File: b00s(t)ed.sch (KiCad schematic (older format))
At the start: 1 part, among them Q1 IRL7472L1

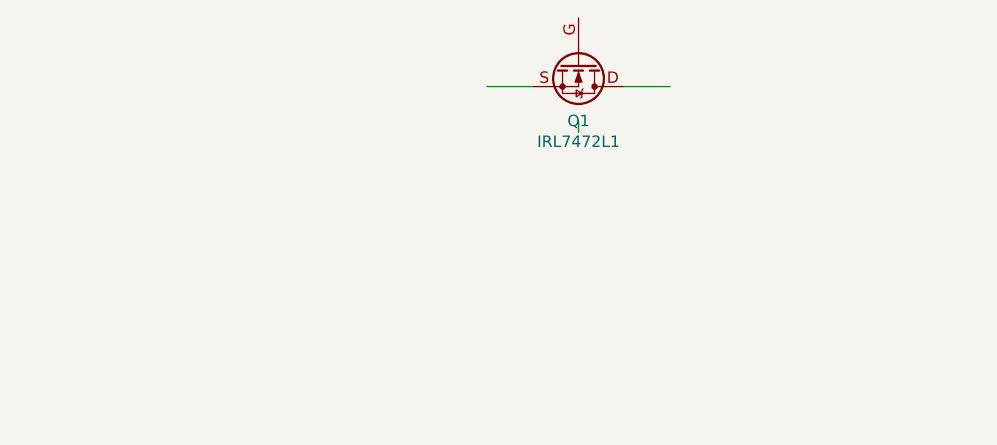
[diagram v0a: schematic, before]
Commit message: backup
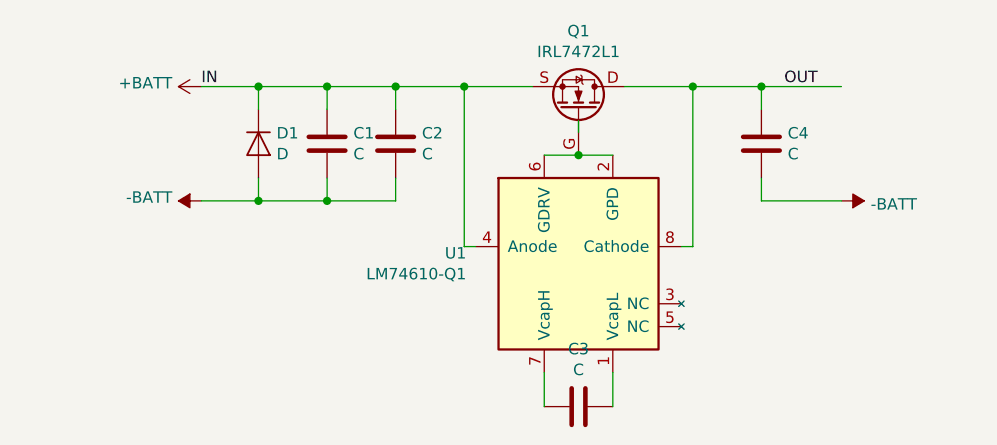
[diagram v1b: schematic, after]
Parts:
- added C1, C2, C3, C4: C, Capacitor_SMD:C_1206_3216Metric, symbol Device:C
- added D1: D, Diode_SMD:D_SMB, symbol Device:D
- added U1: LM74610-Q1, Package_SO:S-PDSO-G8, symbol Power_Management:LM74610-Q1
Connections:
- net labels added: +BATT, -BATT, IN, OUT
- wire segments 3 -> 29
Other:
- moved on the sheet: Q1
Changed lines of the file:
@@
 $EndDescr
 Wire Wire Line
-	5700 2400 5500 2400
+	5700 2400 5400 2400
 Wire Wire Line
 	5900 2600 5900 2550
@@
 L Transistor_FET:IRL7472L1 Q1
 U 1 1 5C52EA7D
-P 5900 2300
-F 0 "Q1" V 6150 2300 50  0000 C CNN
-F 1 "IRL7472L1" V 6241 2300 50  0000 C CNN
-F 2 "Package_DirectFET:DirectFET_L8" H 5900 2300 50  0001 C CIN
-F 3 "https://www.infineon.com/dgdl/Infineon-IRL7472L1-DS-v02_00-EN.pdf?fileId=5546d46254e133b401555d17178250d8" H 5900 2300 50  0001 L CNN
-	1    5900 2300
+P 5900 2500
+F 0 "Q1" V 6243 2500 50  0000 C CNN
+F 1 "IRL7472L1" V 6152 2500 50  0000 C CNN
+F 2 "Package_DirectFET:DirectFET_L8" H 5900 2500 50  0001 C CIN
+F 3 "https://www.infineon.com/dgdl/Infineon-IRL7472L1-DS-v02_00-EN.pdf?fileId=5546d46254e133b401555d17178250d8" H 5900 2500 50  0001 L CNN
+	1    5900 2500
+	0    1    -1   0
+$EndComp
+Wire Wire Line
+	6100 2400 6400 2400
+Text Label 4250 2400 0    50   ~ 0
+IN
+Text Label 6800 2400 0    50   ~ 0
+OUT
+$Comp
+L Power_Management:LM74610-Q1 U1
+U 1 1 5C5374D8
+P 5900 2950
+F 0 "U1" H 5409 2771 50  0000 R CNN
+F 1 "LM74610-Q1" H 5409 2680 50  0000 R CNN
+F 2 "Package_SO:S-PDSO-G8" H 5900 2250 50  0001 C CIN
+F 3 "http://www.irf.com/product-info/datasheets/data/auips7111s.pdf" H 5900 3150 50  0001 C CNN
+	1    5900 2950
+	1    0    0    -1
+$EndComp
+Wire Wire Line
+	5450 3100 5400 3100
+Wire Wire Line
+	5400 3100 5400 2400
+Connection ~ 5400 2400
+Wire Wire Line
+	5400 2400 5100 2400
+Wire Wire Line
+	6350 3100 6400 3100
+Wire Wire Line
+	6400 3100 6400 2400
+Connection ~ 6400 2400
+Wire Wire Line
+	6400 2400 6700 2400
+Wire Wire Line
+	5750 2700 5900 2700
+Wire Wire Line
+	6050 2700 5900 2700
+Connection ~ 5900 2700
+$Comp
+L Device:C C3
+U 1 1 5C53C78F
+P 5900 3800
+F 0 "C3" V 5648 3800 50  0000 C CNN
+F 1 "C" V 5739 3800 50  0000 C CNN
+F 2 "Capacitor_SMD:C_1206_3216Metric" H 5938 3650 50  0001 C CNN
+F 3 "~" H 5900 3800 50  0001 C CNN
+	1    5900 3800
 	0    1    1    0
 $EndComp
 Wire Wire Line
-	6100 2400 6300 2400
+	6050 3650 6050 3800
+Wire Wire Line
+	5750 3650 5750 3800
+$Comp
+L Device:D D1
+U 1 1 5C53D25D
+P 4500 2650
+F 0 "D1" V 4454 2729 50  0000 L CNN
+F 1 "D" V 4545 2729 50  0000 L CNN
+F 2 "Diode_SMD:D_SMB" H 4500 2650 50  0001 C CNN
+F 3 "~" H 4500 2650 50  0001 C CNN
+	1    4500 2650
+	0    1    1    0
+$EndComp
+$Comp
+L Device:C C2
+U 1 1 5C53D3D8
+P 5100 2650
+F 0 "C2" H 5215 2696 50  0000 L CNN
+F 1 "C" H 5215 2605 50  0000 L CNN
+F 2 "Capacitor_SMD:C_1206_3216Metric" H 5138 2500 50  0001 C CNN
+F 3 "~" H 5100 2650 50  0001 C CNN
+	1    5100 2650
+	1    0    0    -1
+$EndComp
+Wire Wire Line
+	5100 2500 5100 2400
+Connection ~ 5100 2400
+Wire Wire Line
+	5100 2400 4800 2400
+Wire Wire Line
+	4800 2500 4800 2400
+Connection ~ 4800 2400
+Wire Wire Line
+	4800 2400 4500 2400
+$Comp
+L Device:C C4
+U 1 1 5C53E8AA
+P 6700 2650
+F 0 "C4" H 6815 2696 50  0000 L CNN
+F 1 "C" H 6815 2605 50  0000 L CNN
+F 2 "Capacitor_SMD:C_1206_3216Metric" H 6738 2500 50  0001 C CNN
+F 3 "~" H 6700 2650 50  0001 C CNN
+	1    6700 2650
+	1    0    0    -1
+$EndComp
+Wire Wire Line
+	6700 2900 6700 2800
+Wire Wire Line
+	6700 2500 6700 2400
+Connection ~ 6700 2400
+Wire Wire Line
+	6700 2400 7050 2400
+$Comp
+L Device:C C1
+U 1 1 5C54035D
+P 4800 2650
+F 0 "C1" H 4915 2696 50  0000 L CNN
+F 1 "C" H 4915 2605 50  0000 L CNN
+F 2 "Capacitor_SMD:C_1206_3216Metric" H 4838 2500 50  0001 C CNN
+F 3 "~" H 4800 2650 50  0001 C CNN
+	1    4800 2650
+	1    0    0    -1
+$EndComp
+Wire Wire Line
+	4500 2500 4500 2400
+Connection ~ 4500 2400
+Wire Wire Line
+	4500 2400 4250 2400
+$Comp
+L power:+BATT #PWR0101
+U 1 1 5C5419B9
+P 4250 2400
+F 0 "#PWR0101" H 4250 2250 50  0001 C CNN
+F 1 "+BATT" V 4265 2527 50  0000 L CNN
+F 2 "" H 4250 2400 50  0001 C CNN
+F 3 "" H 4250 2400 50  0001 C CNN
+	1    4250 2400
+	0    -1   -1   0
+$EndComp
+$Comp
+L power:-BATT #PWR0103
+U 1 1 5C54344F
+P 4250 2900
+F 0 "#PWR0103" H 4250 2750 50  0001 C CNN
+F 1 "-BATT" V 4265 3027 50  0000 L CNN
+F 2 "" H 4250 2900 50  0001 C CNN
+F 3 "" H 4250 2900 50  0001 C CNN
+	1    4250 2900
+	0    -1   -1   0
+$EndComp
+$Comp
+L power:-BATT #PWR0104
+U 1 1 5C544FA1
+P 7050 2900
+F 0 "#PWR0104" H 7050 2750 50  0001 C CNN
+F 1 "-BATT" V 7065 3028 50  0000 L CNN
+F 2 "" H 7050 2900 50  0001 C CNN
+F 3 "" H 7050 2900 50  0001 C CNN
+	1    7050 2900
+	0    1    1    0
+$EndComp
+Wire Wire Line
+	6700 2900 7050 2900
+Wire Wire Line
+	4250 2900 4500 2900
+Wire Wire Line
+	5100 2900 5100 2800
+Wire Wire Line
+	4800 2800 4800 2900
+Connection ~ 4800 2900
+Wire Wire Line
+	4800 2900 5100 2900
+Wire Wire Line
+	4500 2800 4500 2900
+Connection ~ 4500 2900
+Wire Wire Line
+	4500 2900 4800 2900
 $EndSCHEMATC

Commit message: First version ready for order
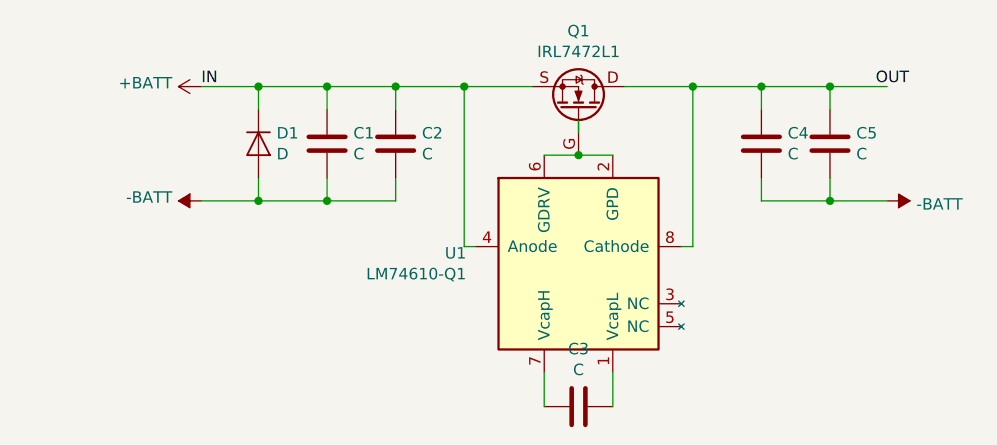
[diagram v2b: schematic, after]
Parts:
- added C5: C, Capacitor_SMD:C_1206_3216Metric, symbol Device:C
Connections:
- wire segments 29 -> 33
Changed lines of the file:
@@
 Text Label 4250 2400 0    50   ~ 0
 IN
-Text Label 6800 2400 0    50   ~ 0
+Text Label 7200 2400 0    50   ~ 0
 OUT
 $Comp
@@
 Connection ~ 6700 2400
 Wire Wire Line
-	6700 2400 7050 2400
+	6700 2400 7000 2400
 $Comp
 L Device:C C1
@@
 L power:-BATT #PWR0104
 U 1 1 5C544FA1
-P 7050 2900
-F 0 "#PWR0104" H 7050 2750 50  0001 C CNN
-F 1 "-BATT" V 7065 3028 50  0000 L CNN
-F 2 "" H 7050 2900 50  0001 C CNN
-F 3 "" H 7050 2900 50  0001 C CNN
-	1    7050 2900
+P 7250 2900
+F 0 "#PWR0104" H 7250 2750 50  0001 C CNN
+F 1 "-BATT" V 7265 3028 50  0000 L CNN
+F 2 "" H 7250 2900 50  0001 C CNN
+F 3 "" H 7250 2900 50  0001 C CNN
+	1    7250 2900
 	0    1    1    0
 $EndComp
 Wire Wire Line
-	6700 2900 7050 2900
+	6700 2900 7000 2900
 Wire Wire Line
 	4250 2900 4500 2900
@@
 Wire Wire Line
 	4500 2900 4800 2900
+$Comp
+L Device:C C5
+U 1 1 5C555923
+P 7000 2650
+F 0 "C5" H 7115 2696 50  0000 L CNN
+F 1 "C" H 7115 2605 50  0000 L CNN
+F 2 "Capacitor_SMD:C_1206_3216Metric" H 7038 2500 50  0001 C CNN
+F 3 "~" H 7000 2650 50  0001 C CNN
+	1    7000 2650
+	1    0    0    -1
+$EndComp
+Wire Wire Line
+	7000 2500 7000 2400
+Connection ~ 7000 2400
+Wire Wire Line
+	7000 2400 7250 2400
+Wire Wire Line
+	7000 2800 7000 2900
+Connection ~ 7000 2900
+Wire Wire Line
+	7000 2900 7250 2900
 $EndSCHEMATC

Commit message: ordered
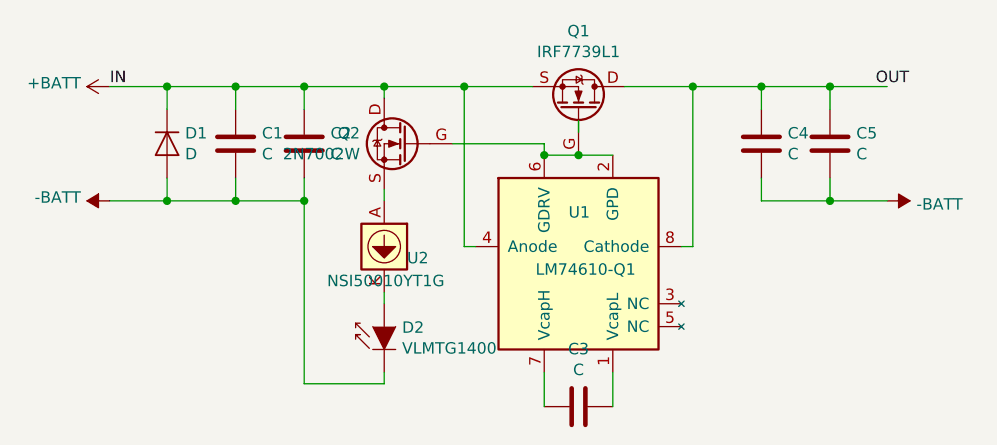
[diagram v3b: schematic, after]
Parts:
- added D2: VLMTG1400, Diode_SMD:D_0603_1608Metric, symbol LED:VLMTG1400
- added Q2: 2N7002W, Package_TO_SOT_SMD:SOT-323_SC-70, symbol Transistor_FET:2N7002W
- added U2: NSI50010YT1G, Digikey:SOD-123, symbol Regulator_Current:NSI50010YT1G
- Q1: value IRL7472L1 -> IRF7739L1
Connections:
- wire segments 33 -> 42
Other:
- moved on the sheet: C1, C2, D1
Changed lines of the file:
@@
 P 5900 2500
 F 0 "Q1" V 6243 2500 50  0000 C CNN
-F 1 "IRL7472L1" V 6152 2500 50  0000 C CNN
+F 1 "IRF7739L1" V 6152 2500 50  0000 C CNN
 F 2 "Package_DirectFET:DirectFET_L8" H 5900 2500 50  0001 C CIN
-F 3 "https://www.infineon.com/dgdl/Infineon-IRL7472L1-DS-v02_00-EN.pdf?fileId=5546d46254e133b401555d17178250d8" H 5900 2500 50  0001 L CNN
+F 3 "" H 5900 2500 50  0001 L CNN
 	1    5900 2500
 	0    1    -1   0
@@
 Wire Wire Line
 	6100 2400 6400 2400
-Text Label 4250 2400 0    50   ~ 0
+Text Label 3850 2400 0    50   ~ 0
 IN
 Text Label 7200 2400 0    50   ~ 0
@@
 U 1 1 5C5374D8
 P 5900 2950
-F 0 "U1" H 5409 2771 50  0000 R CNN
-F 1 "LM74610-Q1" H 5409 2680 50  0000 R CNN
+F 0 "U1" H 5950 2950 50  0000 R CNN
+F 1 "LM74610-Q1" H 6150 2700 50  0000 R CNN
 F 2 "Package_SO:S-PDSO-G8" H 5900 2250 50  0001 C CIN
-F 3 "http://www.irf.com/product-info/datasheets/data/auips7111s.pdf" H 5900 3150 50  0001 C CNN
+F 3 "" H 5900 3150 50  0001 C CNN
 	1    5900 2950
 	1    0    0    -1
@@
 Wire Wire Line
 	5400 3100 5400 2400
-Connection ~ 5400 2400
-Wire Wire Line
-	5400 2400 5100 2400
+Wire Wire Line
+	5400 2400 5050 2400
 Wire Wire Line
 	6350 3100 6400 3100
@@
 F 1 "C" V 5739 3800 50  0000 C CNN
 F 2 "Capacitor_SMD:C_1206_3216Metric" H 5938 3650 50  0001 C CNN
-F 3 "~" H 5900 3800 50  0001 C CNN
+F 3 "" H 5900 3800 50  0001 C CNN
 	1    5900 3800
 	0    1    1    0
@@
 L Device:D D1
 U 1 1 5C53D25D
-P 4500 2650
-F 0 "D1" V 4454 2729 50  0000 L CNN
-F 1 "D" V 4545 2729 50  0000 L CNN
-F 2 "Diode_SMD:D_SMB" H 4500 2650 50  0001 C CNN
-F 3 "~" H 4500 2650 50  0001 C CNN
-	1    4500 2650
+P 4100 2650
+F 0 "D1" V 4054 2729 50  0000 L CNN
+F 1 "D" V 4145 2729 50  0000 L CNN
+F 2 "Diode_SMD:D_SMB" H 4100 2650 50  0001 C CNN
+F 3 "" H 4100 2650 50  0001 C CNN
+	1    4100 2650
 	0    1    1    0
 $EndComp
@@
 L Device:C C2
 U 1 1 5C53D3D8
-P 5100 2650
-F 0 "C2" H 5215 2696 50  0000 L CNN
-F 1 "C" H 5215 2605 50  0000 L CNN
-F 2 "Capacitor_SMD:C_1206_3216Metric" H 5138 2500 50  0001 C CNN
-F 3 "~" H 5100 2650 50  0001 C CNN
-	1    5100 2650
-	1    0    0    -1
-$EndComp
-Wire Wire Line
-	5100 2500 5100 2400
-Connection ~ 5100 2400
-Wire Wire Line
-	5100 2400 4800 2400
-Wire Wire Line
-	4800 2500 4800 2400
-Connection ~ 4800 2400
-Wire Wire Line
-	4800 2400 4500 2400
+P 4700 2650
+F 0 "C2" H 4815 2696 50  0000 L CNN
+F 1 "C" H 4815 2605 50  0000 L CNN
+F 2 "Capacitor_SMD:C_1206_3216Metric" H 4738 2500 50  0001 C CNN
+F 3 "" H 4700 2650 50  0001 C CNN
+	1    4700 2650
+	1    0    0    -1
+$EndComp
+Wire Wire Line
+	4700 2500 4700 2400
+Connection ~ 4700 2400
+Wire Wire Line
+	4700 2400 4400 2400
+Wire Wire Line
+	4400 2500 4400 2400
+Connection ~ 4400 2400
+Wire Wire Line
+	4400 2400 4100 2400
 $Comp
 L Device:C C4
@@
 F 1 "C" H 6815 2605 50  0000 L CNN
 F 2 "Capacitor_SMD:C_1206_3216Metric" H 6738 2500 50  0001 C CNN
-F 3 "~" H 6700 2650 50  0001 C CNN
+F 3 "" H 6700 2650 50  0001 C CNN
 	1    6700 2650
 	1    0    0    -1
@@
 L Device:C C1
 U 1 1 5C54035D
-P 4800 2650
-F 0 "C1" H 4915 2696 50  0000 L CNN
-F 1 "C" H 4915 2605 50  0000 L CNN
-F 2 "Capacitor_SMD:C_1206_3216Metric" H 4838 2500 50  0001 C CNN
-F 3 "~" H 4800 2650 50  0001 C CNN
-	1    4800 2650
-	1    0    0    -1
-$EndComp
-Wire Wire Line
-	4500 2500 4500 2400
-Connection ~ 4500 2400
-Wire Wire Line
-	4500 2400 4250 2400
+P 4400 2650
+F 0 "C1" H 4515 2696 50  0000 L CNN
+F 1 "C" H 4515 2605 50  0000 L CNN
+F 2 "Capacitor_SMD:C_1206_3216Metric" H 4438 2500 50  0001 C CNN
+F 3 "" H 4400 2650 50  0001 C CNN
+	1    4400 2650
+	1    0    0    -1
+$EndComp
+Wire Wire Line
+	4100 2500 4100 2400
+Connection ~ 4100 2400
+Wire Wire Line
+	4100 2400 3850 2400
 $Comp
 L power:+BATT #PWR0101
 U 1 1 5C5419B9
-P 4250 2400
-F 0 "#PWR0101" H 4250 2250 50  0001 C CNN
-F 1 "+BATT" V 4265 2527 50  0000 L CNN
-F 2 "" H 4250 2400 50  0001 C CNN
-F 3 "" H 4250 2400 50  0001 C CNN
-	1    4250 2400
+P 3850 2400
+F 0 "#PWR0101" H 3850 2250 50  0001 C CNN
+F 1 "+BATT" V 3865 2527 50  0000 L CNN
+F 2 "" H 3850 2400 50  0001 C CNN
+F 3 "" H 3850 2400 50  0001 C CNN
+	1    3850 2400
 	0    -1   -1   0
 $EndComp
@@
 L power:-BATT #PWR0103
 U 1 1 5C54344F
-P 4250 2900
-F 0 "#PWR0103" H 4250 2750 50  0001 C CNN
-F 1 "-BATT" V 4265 3027 50  0000 L CNN
-F 2 "" H 4250 2900 50  0001 C CNN
-F 3 "" H 4250 2900 50  0001 C CNN
-	1    4250 2900
+P 3850 2900
+F 0 "#PWR0103" H 3850 2750 50  0001 C CNN
+F 1 "-BATT" V 3865 3027 50  0000 L CNN
+F 2 "" H 3850 2900 50  0001 C CNN
+F 3 "" H 3850 2900 50  0001 C CNN
+	1    3850 2900
 	0    -1   -1   0
 $EndComp
@@
 	6700 2900 7000 2900
 Wire Wire Line
-	4250 2900 4500 2900
-Wire Wire Line
-	5100 2900 5100 2800
-Wire Wire Line
-	4800 2800 4800 2900
-Connection ~ 4800 2900
-Wire Wire Line
-	4800 2900 5100 2900
-Wire Wire Line
-	4500 2800 4500 2900
-Connection ~ 4500 2900
-Wire Wire Line
-	4500 2900 4800 2900
+	3850 2900 4100 2900
+Wire Wire Line
+	4700 2900 4700 2800
+Wire Wire Line
+	4400 2800 4400 2900
+Connection ~ 4400 2900
+Wire Wire Line
+	4400 2900 4700 2900
+Wire Wire Line
+	4100 2800 4100 2900
+Connection ~ 4100 2900
+Wire Wire Line
+	4100 2900 4400 2900
 $Comp
 L Device:C C5
@@
 F 1 "C" H 7115 2605 50  0000 L CNN
 F 2 "Capacitor_SMD:C_1206_3216Metric" H 7038 2500 50  0001 C CNN
-F 3 "~" H 7000 2650 50  0001 C CNN
+F 3 "" H 7000 2650 50  0001 C CNN
 	1    7000 2650
 	1    0    0    -1
@@
 Wire Wire Line
 	7000 2900 7250 2900
+$Comp
+L Regulator_Current:NSI50010YT1G U2
+U 1 1 5C55B031
+P 5050 3100
+F 0 "U2" V 5100 3200 50  0000 L CNN
+F 1 "NSI50010YT1G" V 5200 2850 50  0000 L CNN
+F 2 "Digikey:SOD-123" H 5050 2800 50  0001 C CNN
+F 3 "https://www.onsemi.com/pub/Collateral/NSI50010Y-D.PDF" H 5050 3100 50  0001 C CNN
+	1    5050 3100
+	0    1    1    0
+$EndComp
+$Comp
+L LED:VLMTG1400 D2
+U 1 1 5C55DD63
+P 5050 3450
+F 0 "D2" V 5046 3372 50  0000 R CNN
+F 1 "VLMTG1400" V 4955 3372 50  0000 R CNN
+F 2 "Diode_SMD:D_0603_1608Metric" H 5050 3625 50  0001 C CNN
+F 3 "http://www.vishay.com/docs/84393/vlmtg1400.pdf" H 5000 3450 50  0001 C CNN
+	1    5050 3450
+	0    -1   -1   0
+$EndComp
+Connection ~ 5400 2400
+Wire Wire Line
+	5050 2400 5050 2450
+Wire Wire Line
+	5050 2400 4700 2400
+Wire Wire Line
+	5050 2850 5050 2900
+Wire Wire Line
+	5050 3300 5050 3350
+Wire Wire Line
+	5050 3650 5050 3700
+Wire Wire Line
+	5050 3700 4700 3700
+Wire Wire Line
+	4700 3700 4700 2900
+Connection ~ 4700 2900
+Connection ~ 5050 2400
+Wire Wire Line
+	5750 2700 5750 2650
+Wire Wire Line
+	5750 2650 5350 2650
+Connection ~ 5750 2700
+$Comp
+L Transistor_FET:2N7002W Q2
+U 1 1 5C56F591
+P 5150 2650
+F 0 "Q2" H 5356 2696 50  0000 L CNN
+F 1 "2N7002W" H 5356 2605 50  0000 L CNN
+F 2 "Package_TO_SOT_SMD:SOT-323_SC-70" H 5350 2575 50  0001 L CIN
+F 3 "https://www.onsemi.com/pub/Collateral/2N7002W-D.PDF" H 5350 2725 50  0001 L CNN
+	1    5150 2650
+	-1   0    0    -1
+$EndComp
 $EndSCHEMATC
